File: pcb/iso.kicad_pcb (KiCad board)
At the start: 2 copper layers, 27.5 x 40.3 mm, 21 parts, among them J1 Conn_01x06, U1 ATmega328P-AU, U2 SRV05-4, X1 Crystal_GND24_Small

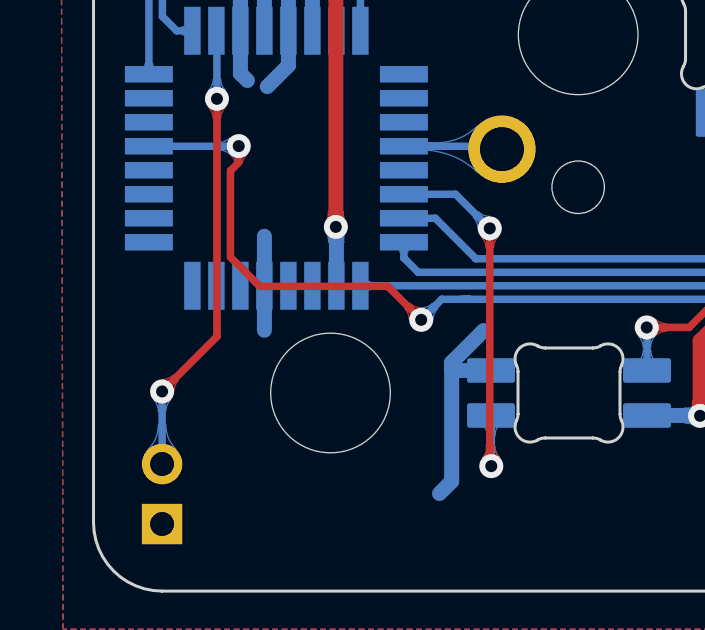
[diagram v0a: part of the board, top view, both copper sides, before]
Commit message: update
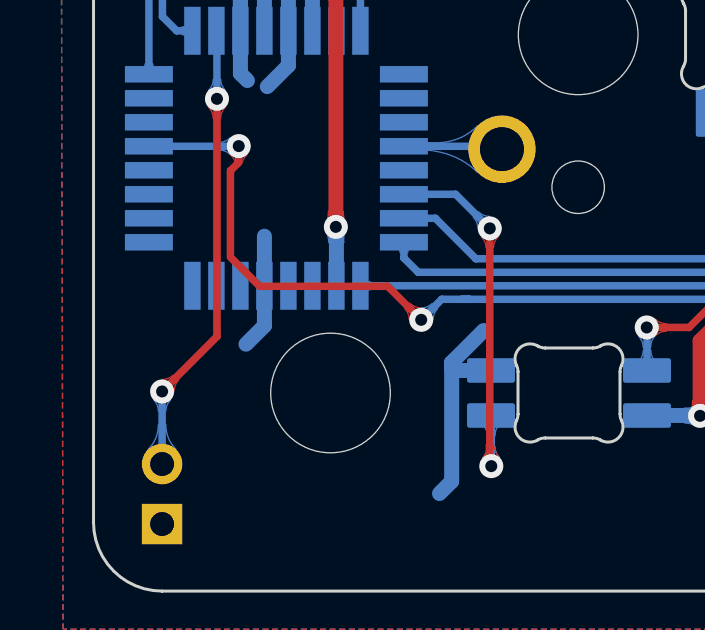
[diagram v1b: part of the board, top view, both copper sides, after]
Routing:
- net GND: track 32.8 -> 33.5 mm
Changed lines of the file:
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@@
     (thickness 1.6)
     (drawings 46)
-    (tracks 231)
+    (tracks 232)
     (zones 0)
     (modules 21)
@@
   (segment (start 147.7708 83.888) (end 147.7708 82.2896) (width 0.5) (layer B.Cu) (net 1))
   (segment (start 146.9708 92.388) (end 146.9708 90.7352) (width 0.5) (layer B.Cu) (net 1))
-  (segment (start 146.9708 92.388) (end 146.9708 93.872) (width 0.5) (layer B.Cu) (net 1))
   (segment (start 146.1708 83.888) (end 146.1708 81.5024) (width 0.5) (layer B.Cu) (net 1))
   (segment (start 147.7708 83.888) (end 147.7708 85.0456) (width 0.5) (layer B.Cu) (net 1))
@@
   (segment (start 142.7988 72.2036) (end 142.7988 71.1708) (width 0.5) (layer B.Cu) (net 1))
   (segment (start 144.8816 72.2036) (end 145.7112 72.2036) (width 0.5) (layer B.Cu) (net 1))
+  (segment (start 146.9708 92.388) (end 146.9708 93.7196) (width 0.5) (layer B.Cu) (net 1))
+  (segment (start 146.9708 93.7196) (end 146.3548 94.3356) (width 0.5) (layer B.Cu) (net 1))
   (segment (start 146.9708 83.888) (end 146.9708 81.9848) (width 0.5) (layer B.Cu) (net 2))
   (segment (start 146.9708 81.9848) (end 147.7772 81.1784) (width 0.5) (layer B.Cu) (net 2))

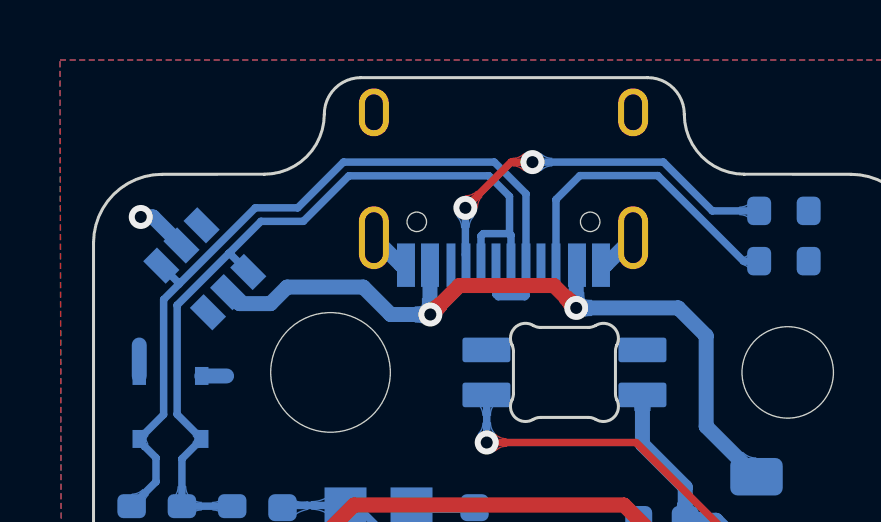
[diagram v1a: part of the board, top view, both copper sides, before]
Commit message: update
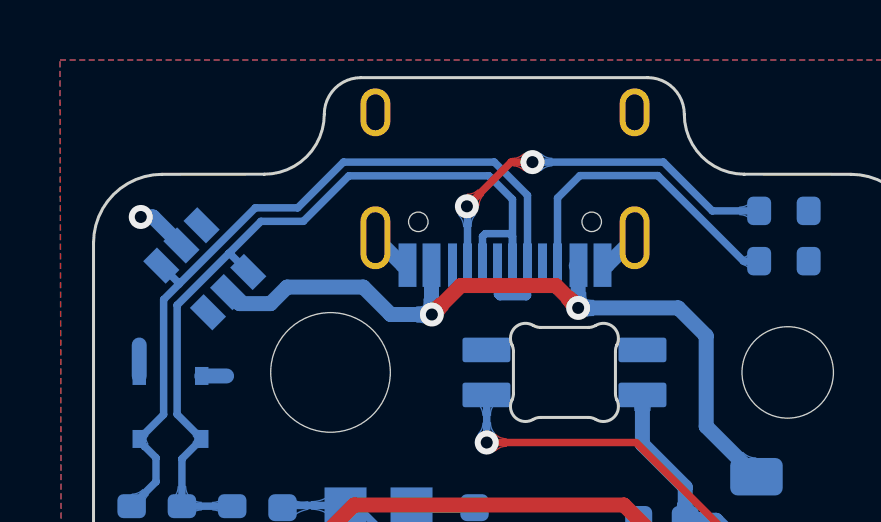
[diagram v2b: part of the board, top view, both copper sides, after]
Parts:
- moved USB1 0.05 mm to (155.0, 64.5)
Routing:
- net Net-(D1-Pad1): track 27.3 -> 28.4 mm
